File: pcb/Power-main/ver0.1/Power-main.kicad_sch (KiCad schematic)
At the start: 2 parts, among them U1 LM5143QRHARQ1, U2 TPS54335ADDAR

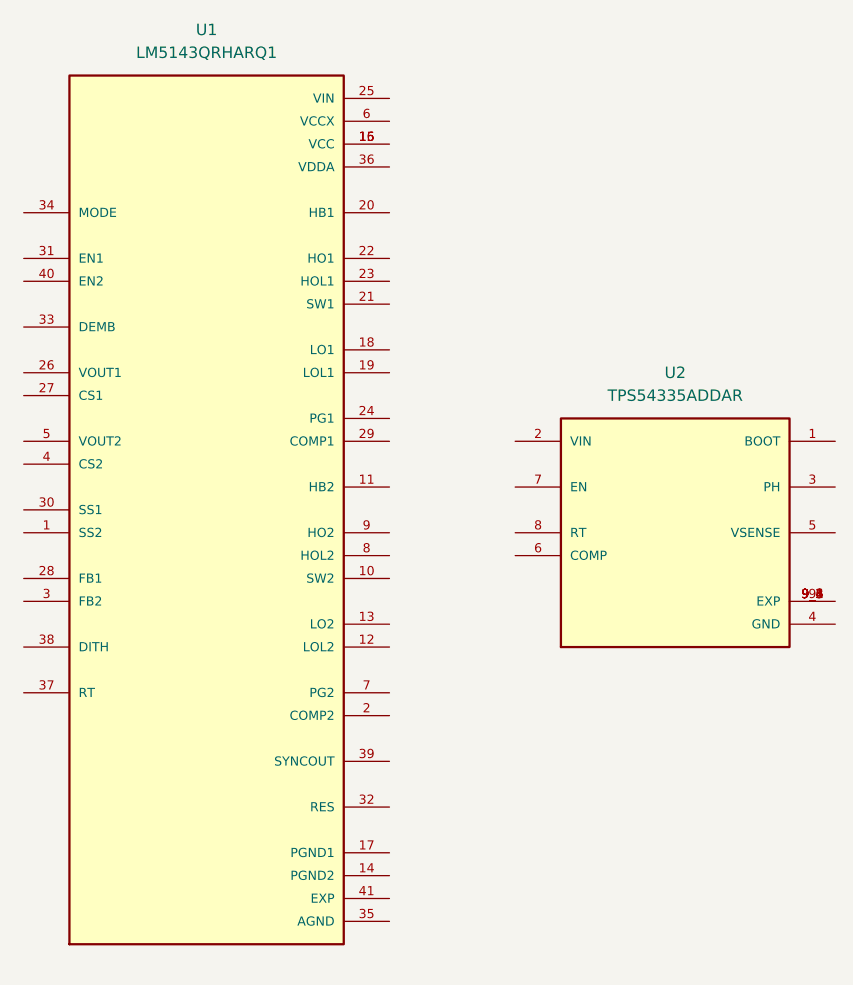
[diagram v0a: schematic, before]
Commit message: dally upload
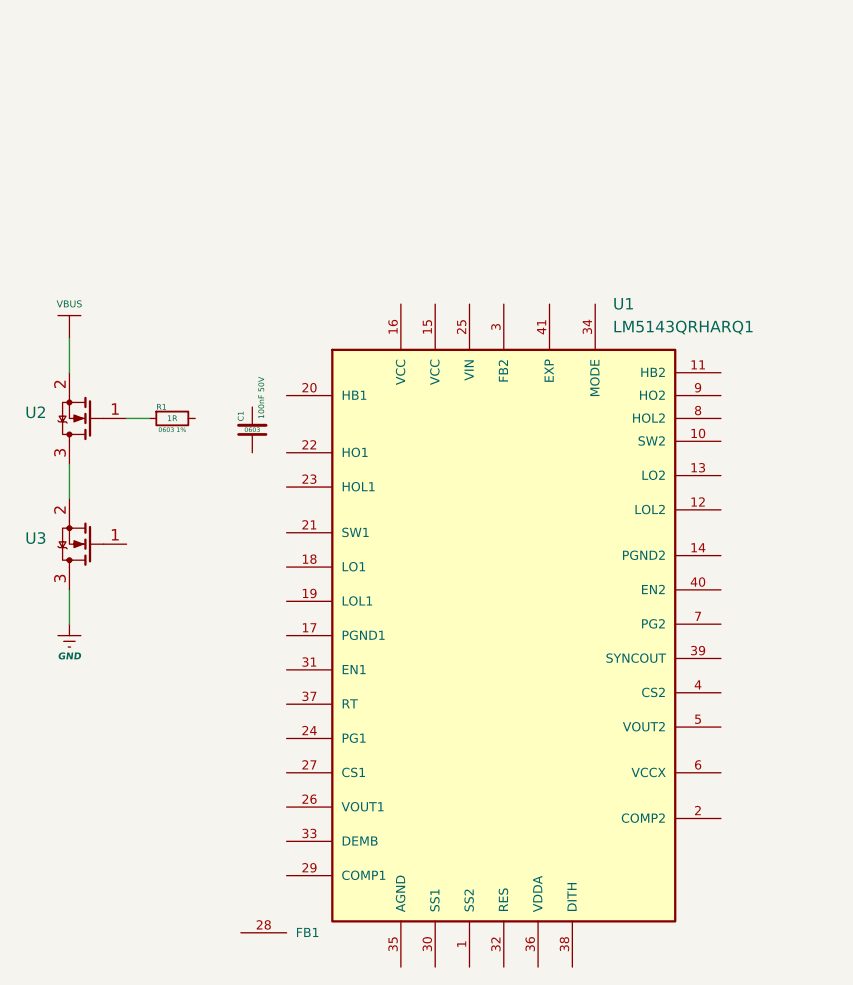
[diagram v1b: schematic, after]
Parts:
- removed U2: TPS54335ADDAR, BuckConvert:TPS54335ADDAR, symbol BuckConvert:TPS54335ADDAR
- added C1: ~, Capacitor_SMD:C_0603_1608Metric, symbol Capacitor:C0603
- added R1: ~, Resistor_SMD:R_0603_1608Metric, symbol Resistor:R0603
- added U2, U3: ~, symbol MOSFET_Channel-N:Symbol-NMOS
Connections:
- net at U1.15 (VCC): no longer U1.16 (VCC)
- new net: U2.3, U3.2
- new net: R1.1, U2.1
- new net GND: U3.3
- new net VBUS: U2.2
